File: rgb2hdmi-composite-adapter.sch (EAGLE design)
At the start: 24 parts

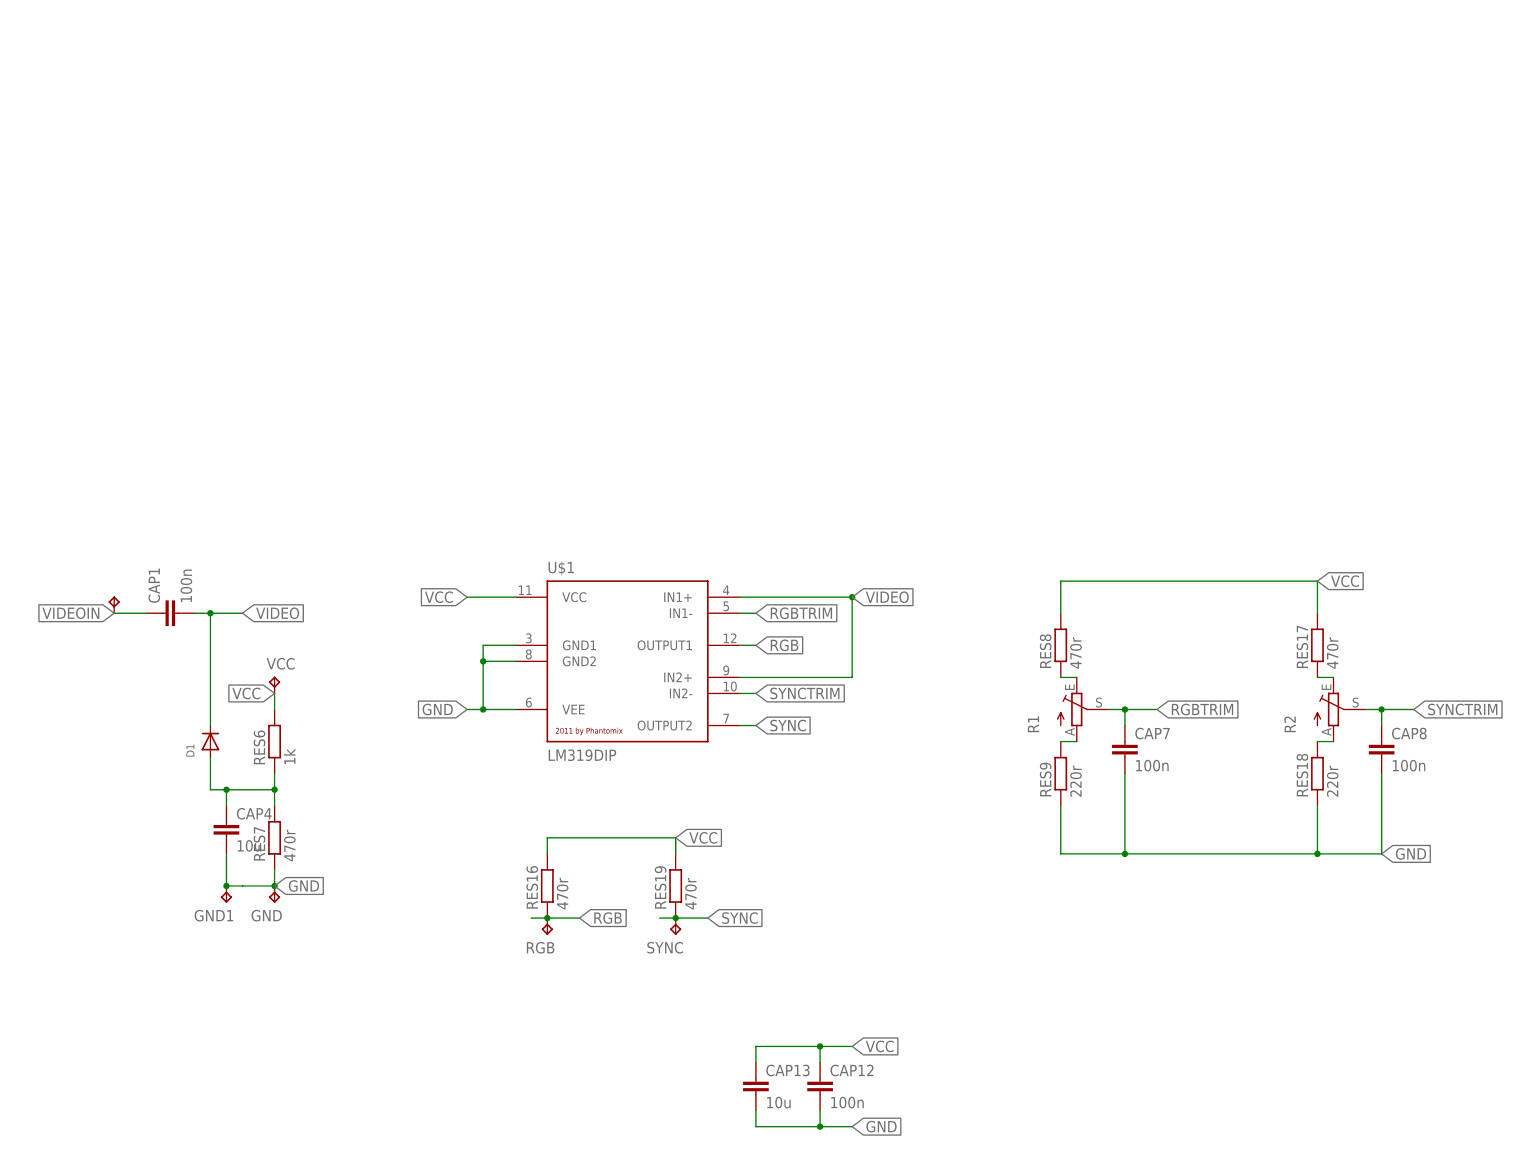
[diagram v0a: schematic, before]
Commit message: update design
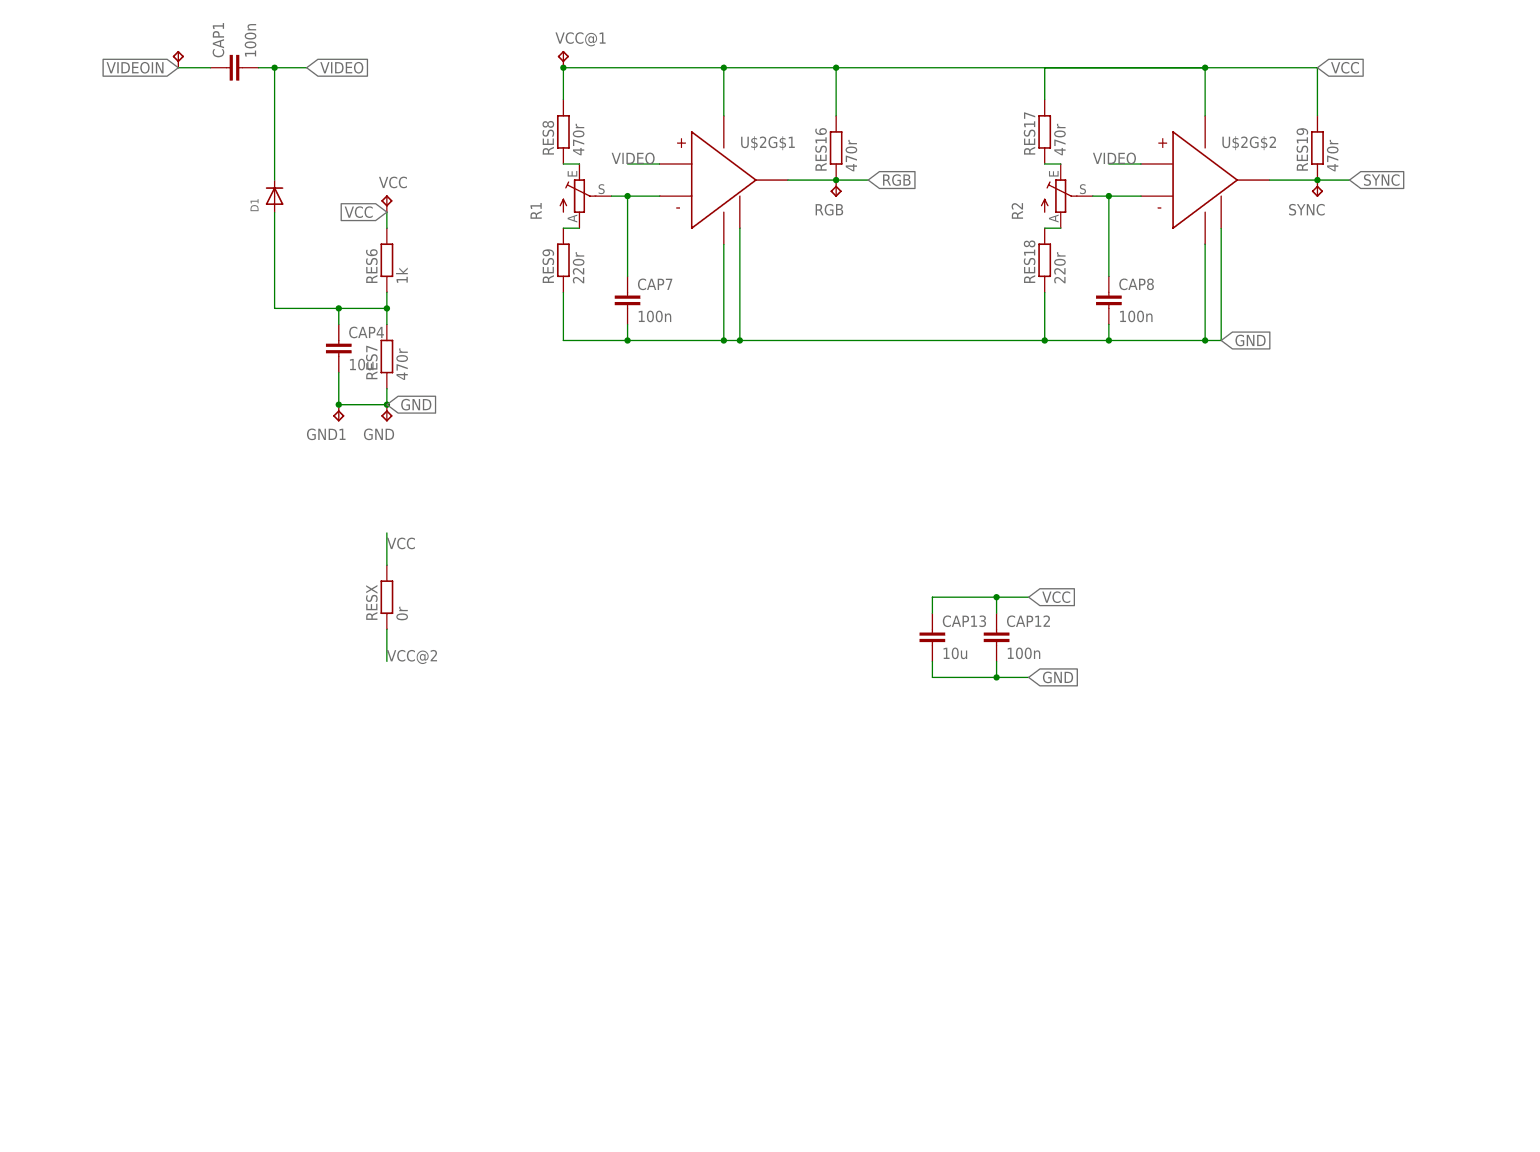
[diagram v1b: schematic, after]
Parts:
- removed U$1: LM319DIP, phantomix-lm319:LM319DIP
- added RESX: 0r, rcl:R-EU_0207/10
- added U$2: LM319, LM319:LM319
- added VCC@1: TPPAD1-17Y, testpad:TPPAD1-17Y
- R1, R2: device pot:TRIM_EU-CA6V -> pot:TRIM_EU-B64Y
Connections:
- new net VCC@2: RESX.1
- net GND: now also U$2G$1.GND, U$2G$1.GND2, U$2G$2.GND, U$2G$2.GND2; no longer U$1.GND1, U$1.GND2, U$1.VEE
- net RGB: now also U$2G$1.OUT; no longer U$1.OUTPUT1
- net RGBTRIM: now also U$2G$1.INV; no longer U$1.IN1-
- net SYNC: now also U$2G$2.OUT; no longer U$1.OUTPUT2
- net SYNCTRIM: now also U$2G$2.INV; no longer U$1.IN2-
- net VCC: now also RESX.2, U$2G$1.VCC, U$2G$2.VCC, VCC@1.TP; no longer U$1.VCC
- net VIDEO: now also U$2G$1.NONINV, U$2G$2.NONINV; no longer U$1.IN1+, U$1.IN2+
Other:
- moved on the sheet: CAP1, CAP12, CAP13, CAP4, CAP7, CAP8, D1, GND, GND1, R1, R2, RES16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
